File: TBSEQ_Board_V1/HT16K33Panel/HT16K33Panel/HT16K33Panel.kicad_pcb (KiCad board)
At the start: 2 copper layers, 200 x 90 mm, 85 parts, among them IC1 HT16K33_28SOP-A_, J1 Conn_01x05_Pin

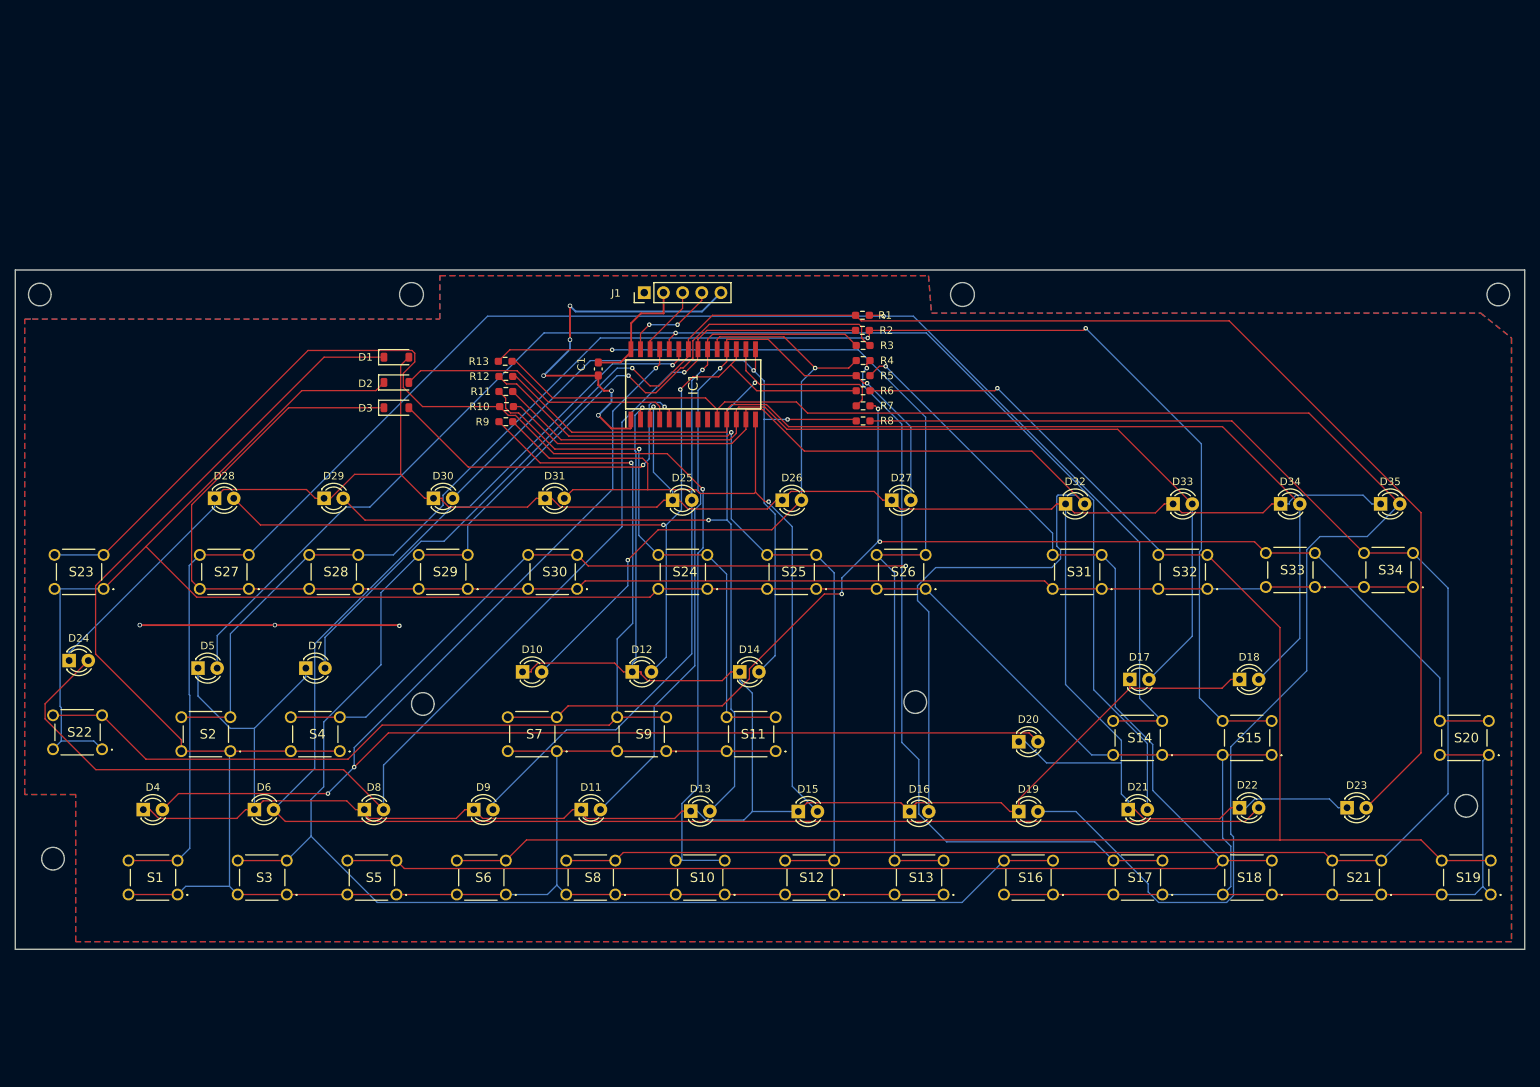
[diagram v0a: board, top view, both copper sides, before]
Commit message: HT16K33 Control
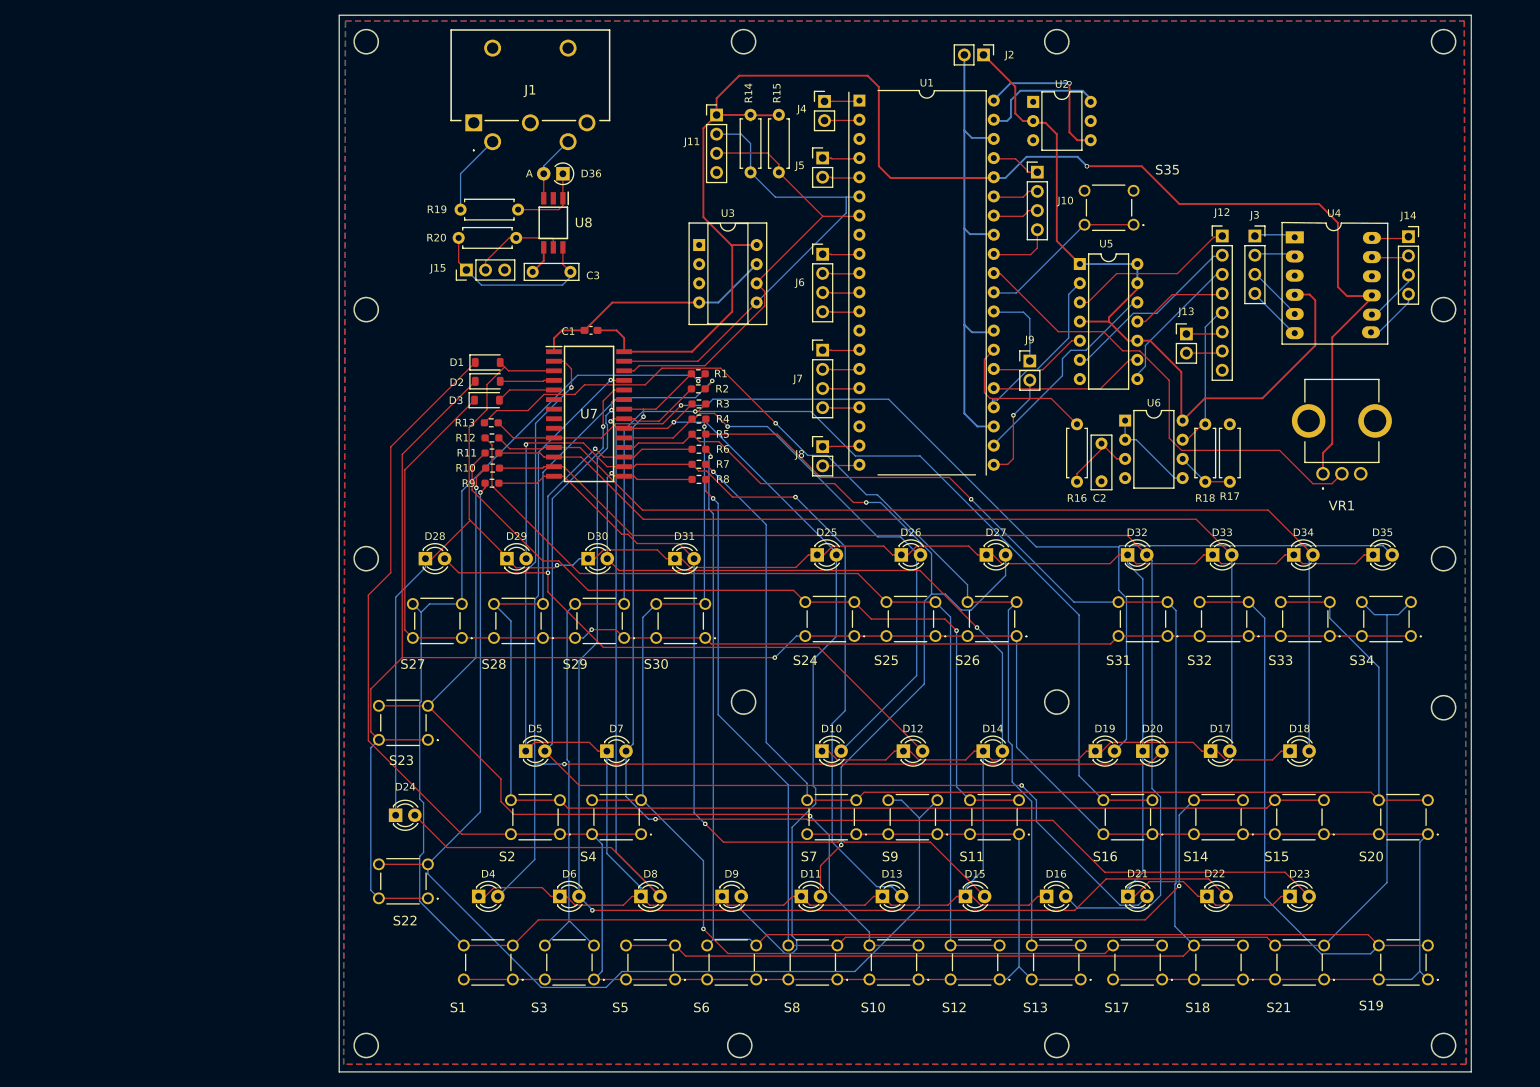
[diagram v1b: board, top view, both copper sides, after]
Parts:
- added C2: 0.047uF, Capacitor_THT:C_Rect_L7.0mm_W2.5mm_P5.00mm, F.Cu at (167.9, 75.8)
- added C3: 0.1uF, Capacitor_THT:C_Rect_L7.0mm_W2.0mm_P5.00mm, F.Cu at (97.6, 53.0)
- added D36: 1SS120TD, Diode_THT:D_A-405_P2.54mm_Vertical_AnodeUp, F.Cu at (96.6, 40.0)
- added J10: Conn_01x04_Socket, Connector_PinHeader_2.54mm:PinHeader_1x04_P2.54mm_Vertical, F.Cu at (159.4, 39.8)
- added J11: Conn_01x04_Socket, Connector_PinHeader_2.54mm:PinHeader_1x04_P2.54mm_Vertical, F.Cu at (116.9, 32.2)
- added J12: Conn_01x08_Pin, Connector_PinHeader_2.54mm:PinHeader_1x08_P2.54mm_Vertical, F.Cu at (183.9, 48.2)
- added J13: Conn_01x02_Pin, Connector_PinHeader_2.54mm:PinHeader_1x02_P2.54mm_Vertical, F.Cu at (179.2, 61.2)
- added J14: Conn_01x04_Pin, Connector_PinSocket_2.54mm:PinSocket_1x04_P2.54mm_Vertical, F.Cu at (208.6, 48.3)
- added J15: Conn_01x03_Pin, Connector_PinHeader_2.54mm:PinHeader_1x03_P2.54mm_Vertical, F.Cu at (83.8, 52.8)
- added J2: Conn_01x02_Socket, Connector_PinHeader_2.54mm:PinHeader_1x02_P2.54mm_Vertical, F.Cu at (152.3, 24.2)
- added J3: Conn_01x04_Pin, Connector_PinSocket_2.54mm:PinSocket_1x04_P2.54mm_Vertical, F.Cu at (188.2, 48.2)
- added J4: Conn_01x02_Pin, Connector_PinHeader_2.54mm:PinHeader_1x02_P2.54mm_Vertical, F.Cu at (131.2, 30.4)
- added J5: Conn_01x02_Pin, Connector_PinHeader_2.54mm:PinHeader_1x02_P2.54mm_Vertical, F.Cu at (131.0, 37.9)
- added J6: Conn_01x04_Socket, Connector_PinHeader_2.54mm:PinHeader_1x04_P2.54mm_Vertical, F.Cu at (131.0, 50.7)
- added J7: Conn_01x04_Socket, Connector_PinHeader_2.54mm:PinHeader_1x04_P2.54mm_Vertical, F.Cu at (131.0, 63.4)
- added J8: Conn_01x02_Pin, Connector_PinHeader_2.54mm:PinHeader_1x02_P2.54mm_Vertical, F.Cu at (131.0, 76.2)
- added J9: Conn_01x02_Pin, Connector_PinHeader_2.54mm:PinHeader_1x02_P2.54mm_Vertical, F.Cu at (158.4, 64.8)
- added R14: 1K, Resistor_THT:R_Axial_DIN0207_L6.3mm_D2.5mm_P7.62mm_Horizontal, F.Cu at (121.4, 32.2)
- added R15: 1K, Resistor_THT:R_Axial_DIN0207_L6.3mm_D2.5mm_P7.62mm_Horizontal, F.Cu at (125.2, 32.2)
- added R16: 22K, Resistor_THT:R_Axial_DIN0207_L6.3mm_D2.5mm_P7.62mm_Horizontal, F.Cu at (164.7, 73.2)
- added R17: 10K, Resistor_THT:R_Axial_DIN0207_L6.3mm_D2.5mm_P7.62mm_Horizontal, F.Cu at (184.9, 80.8)
- added R18: 5.1K, Resistor_THT:R_Axial_DIN0207_L6.3mm_D2.5mm_P7.62mm_Horizontal, F.Cu at (181.7, 80.8)
- added R19: 220, Resistor_THT:R_Axial_DIN0207_L6.3mm_D2.5mm_P7.62mm_Horizontal, F.Cu at (83.0, 44.8)
- added R20: 220, Resistor_THT:R_Axial_DIN0207_L6.3mm_D2.5mm_P7.62mm_Horizontal, F.Cu at (82.8, 48.5)
- added S35: B3F-1000S, SamacSys_Parts:B3F1060, F.Cu at (169.6, 44.5)
- added U1: Raspberry Pi Pico DIP-40, SamacSys_Parts:Raspberry Pi Pico DIP-40_W17.76mm, F.Cu at (144.8, 30.0)
- added U2: IRLML6402(DIP6Convert), Package_DIP:DIP-6_W7.62mm, F.Cu at (158.9, 30.5)
- added U3: FM24CL16B(DIP8 Convert), Package_DIP:CERDIP-8_W7.62mm_SideBrazed_Socket, F.Cu at (114.6, 49.4)
- added U4: AE-LCNV4-MOSFET, SamacSys_Parts:CERDIP-14_W10.16mm_SideBrazed_LongPads_Socket, F.Cu at (198.7, 48.4)
- added U5: 74HC126, Package_DIP:DIP-14_W7.62mm, F.Cu at (165.1, 52.0)
- added U6: LM358, Package_DIP:DIP-8_W7.62mm, F.Cu at (171.1, 72.7)
- added U8: TLP2304_TPR,E, SamacSys_Parts:SOIC127P700X230-6N, F.Cu at (95.3, 46.5)
- added VR1: RK09D117000B, SamacSys_Parts:RK09D117000B, F.Cu at (197.3, 79.8)
- J1: value Conn_01x05_Pin -> KDJ03-5; footprint Connector_PinHeader_2.54mm:PinHeader_1x05_P2.54mm_Vertical -> SamacSys_Parts:KDJ035
- moved D24 47.9 mm to (74.4, 125.0)
- moved S22 47.5 mm to (76.1, 133.8)
- moved S23 47.4 mm to (76.1, 112.8)
- moved D4 45.9 mm to (85.4, 135.8)
- moved S1 45.8 mm to (87.3, 144.5)
- moved S2 45.0 mm to (93.6, 125.2)
- moved D5 44.8 mm to (91.6, 116.5)
- moved S3 42.2 mm to (98.1, 144.5)
- moved D6 42.1 mm to (96.2, 135.8)
- moved S4 41.4 mm to (104.3, 125.2)
- moved D7 41.4 mm to (102.4, 116.5)
- moved S7 41.2 mm to (132.8, 125.2)
- moved D10 41.0 mm to (130.9, 116.5)
- moved S5 38.6 mm to (108.8, 144.5)
- moved D8 38.4 mm to (106.9, 135.8)
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- renumbered IC1 to U7
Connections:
- J1 pad 1: D+5V -> unconnected-(J1-Pad1)
- J1 pad 2: D+3.3V -> unconnected-(J1-Pad2)
- J1 pad 3: D_I2C_SCL -> unconnected-(J1-Pad3)
- J1 pad 4: D_I2C_SDA -> Net-(J1-Pad4)
- J1 pad 5: GNDD -> Net-(D36-A)
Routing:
- net D+3.3V: track 16.3 -> 205.8 mm, vias 0 -> 1
- net D+5V: track 0.00 -> 105.0 mm
- net Row15: track 224.5 -> 158.2 mm, vias 0 -> 1
- net Row3: track 223.2 -> 159.1 mm, vias 1 -> 2
- net Row2: track 221.5 -> 158.5 mm, vias 1 -> 2
- net A+TEMPO: track 0.00 -> 62.8 mm
- net D_I2C_SCL: track 9.29 -> 61.0 mm
- net D_I2C_SDA: track 13.1 -> 64.1 mm, vias 2 -> 0
- net RowK5: track 238.5 -> 187.9 mm
- net Row1: track 192.7 -> 143.3 mm, vias 1 -> 2
- net COM2/KS1: track 353.2 -> 306.4 mm, vias 0 -> 1
- net Row4: track 161.9 -> 115.4 mm
- net RowK6: track 189.9 -> 147.5 mm
- net COM1: track 316.5 -> 275.3 mm
- net RowK10: track 234.4 -> 193.3 mm, vias 0 -> 1
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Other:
- board size 200 x 90 mm -> 150 x 140 mm
